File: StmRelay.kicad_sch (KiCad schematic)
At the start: 8 parts, among them J2 Conn_02x10_Odd_Even, U1 TXS0108EPW, U2 TXS0108EPW

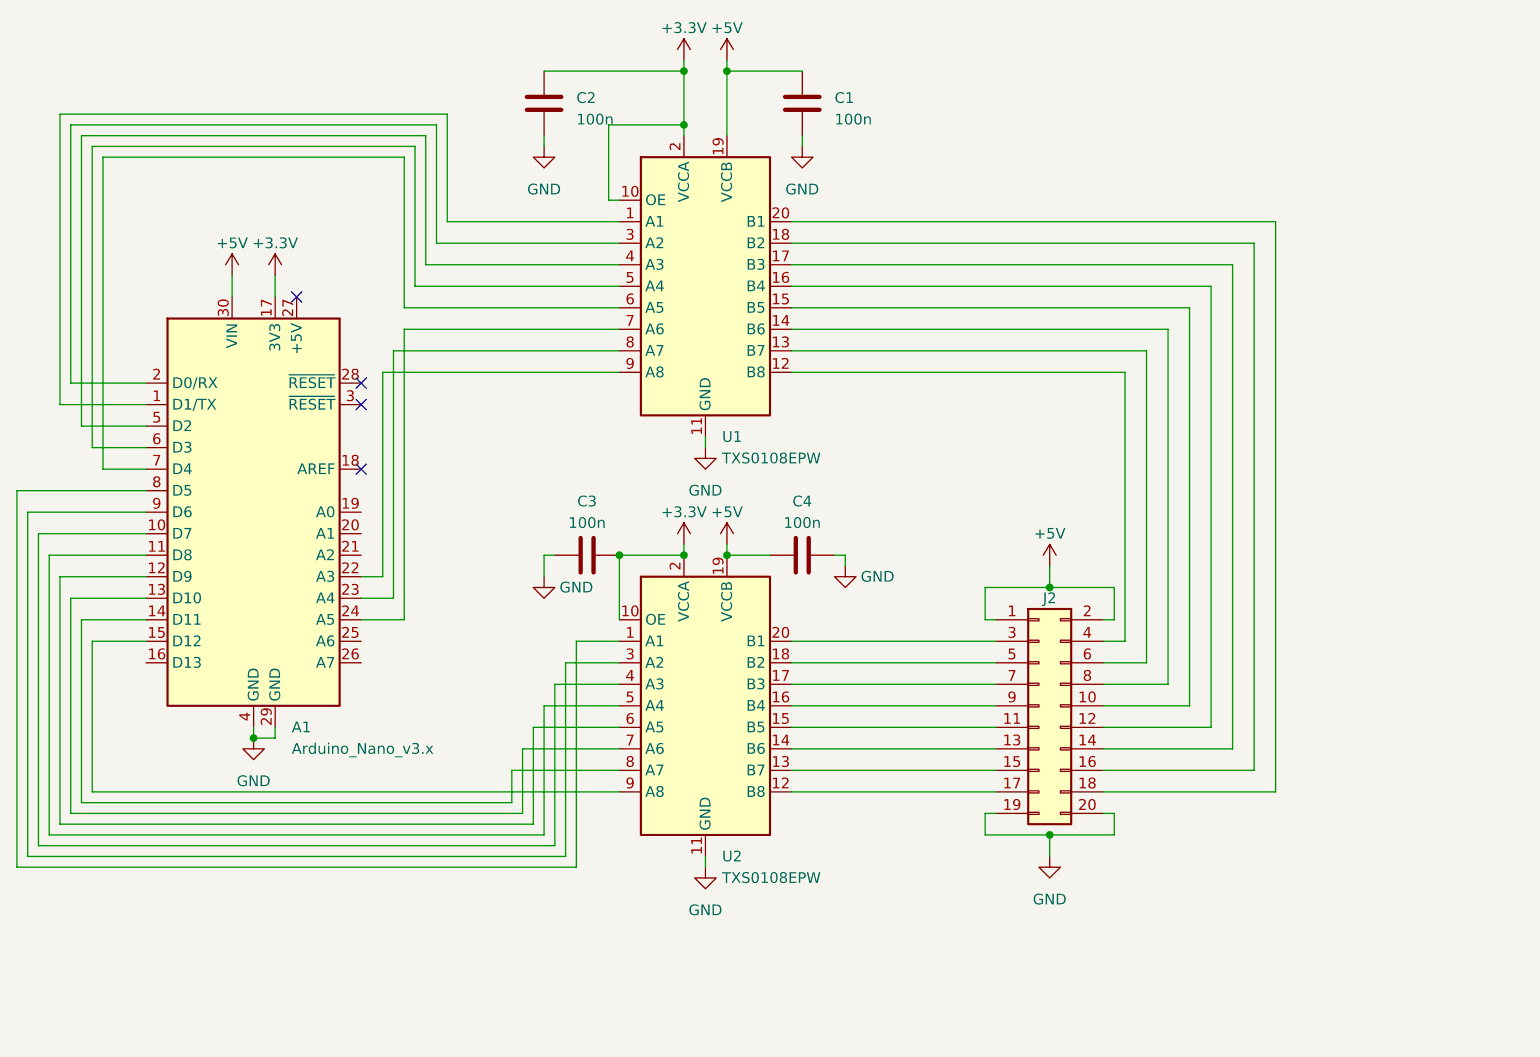
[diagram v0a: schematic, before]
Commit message: last modifs before shipping
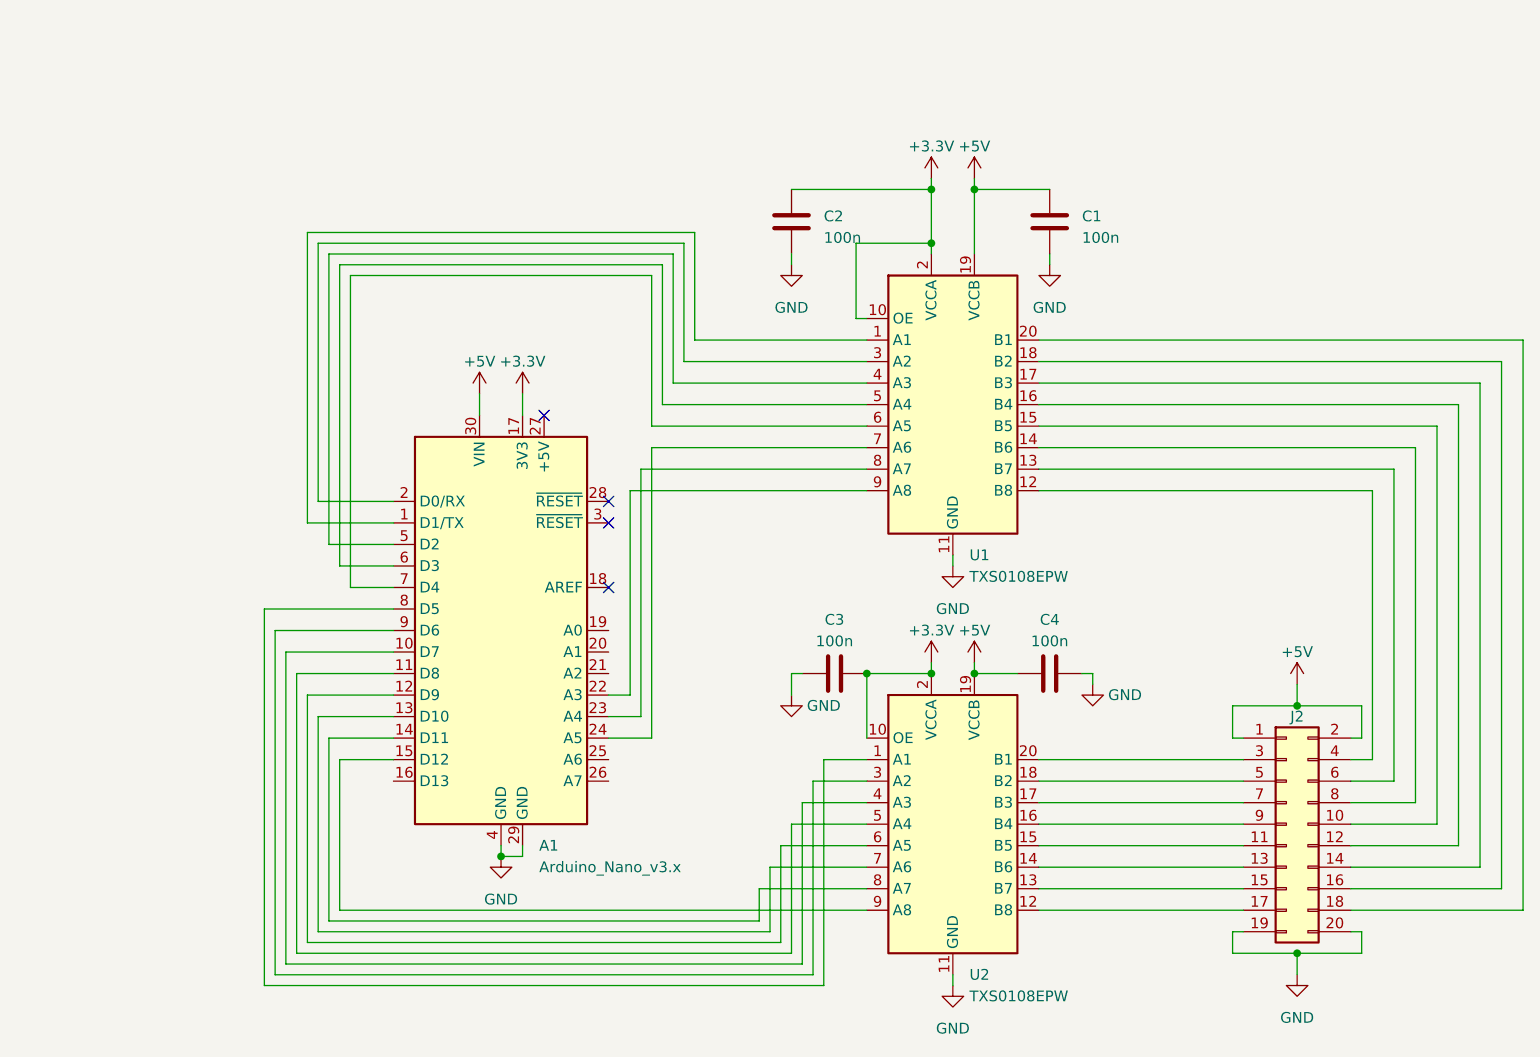
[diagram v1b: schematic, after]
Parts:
- C1, C2, C3, C4: footprint Capacitor_SMD:C_0201_0603Metric -> Capacitor_SMD:C_0603_1608Metric_Pad1.08x0.95mm_HandSolder
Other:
- title: (none) -> STM relay board controller
- moved on the sheet: A1, C1, C2, C3, C4, J2, U1, U2
